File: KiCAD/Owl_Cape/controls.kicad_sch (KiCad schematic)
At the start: 3 parts, among them J17 OLED, SW1 Enter BTN, SW2 Down BTN

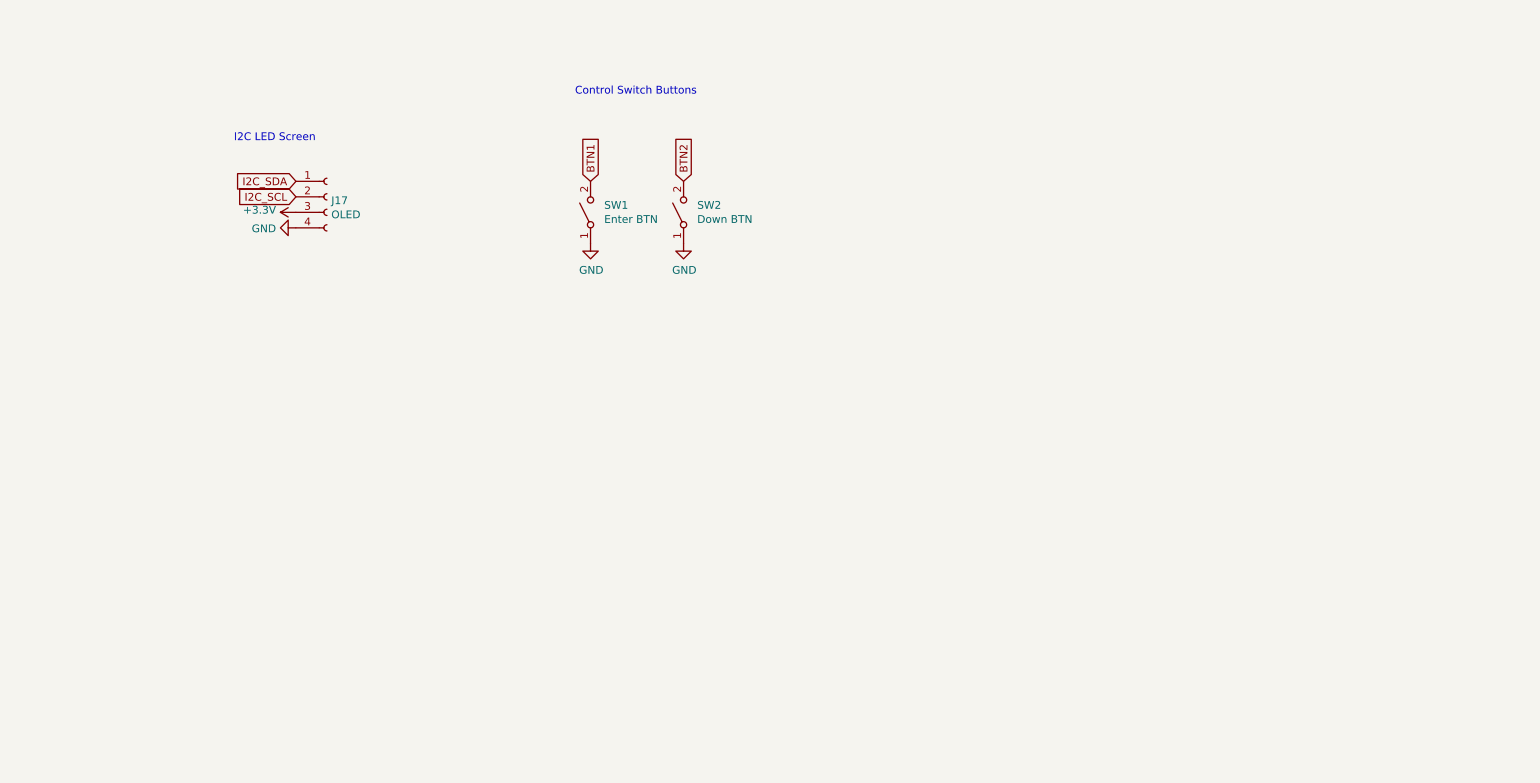
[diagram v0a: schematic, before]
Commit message: started routing cu
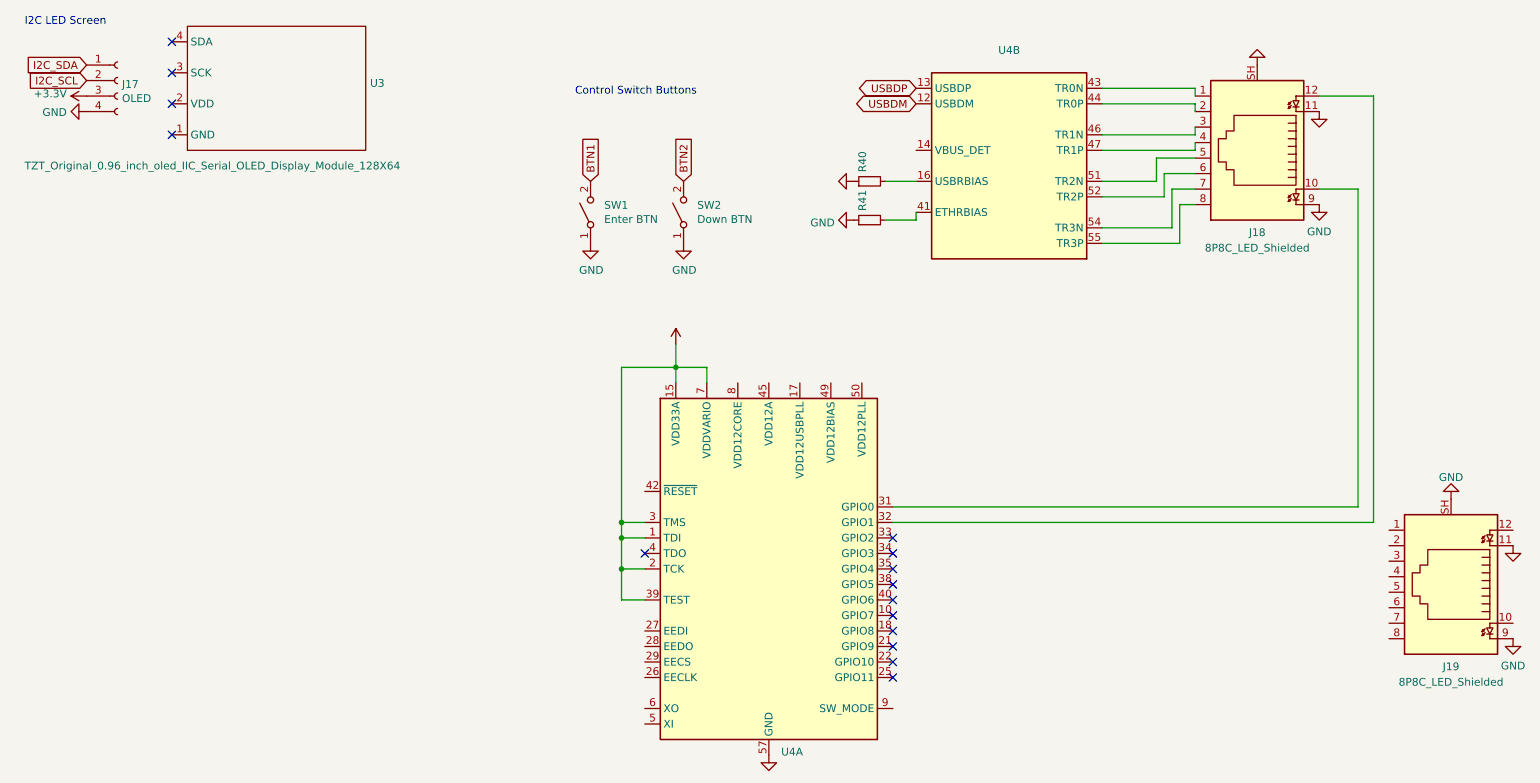
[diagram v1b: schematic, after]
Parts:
- added J18, J19: 8P8C_LED_Shielded, Connector_RJ:RJ45_BEL_SS74301-00x_Vertical, symbol Connector:8P8C_LED_Shielded
- added R40, R41: (no value), symbol Device:R_Small
- added U3: TZT_Original_0.96_inch_oled_IIC_Serial_OLED_Displ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, Stuart_BESPOKE:TZT_0.96inch_OLED, symbol Stuarts_BESPOKE:TZT_Original_0.96_inch_oled_IIC_Serial_OLED_Display_Module_128X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
- added U4: (no value), symbol Interface_Ethernet:LAN7500-ABJZ
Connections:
- net +3V3: now also U4.1 (TDI), U4.15 (VDD33A), U4.19 (VDDVARIO), U4.2 (TCK), U4.24 (VDDVARIO), U4.3 (TMS), U4.37 (VDDVARIO), U4.39 (TEST), U4.7 (VDDVARIO)
- net GND: now also J18.11, J18.9, J18.SH, J19.11, J19.9, J19.SH, R40.1, R41.1, U4.57 (GND)
- new net: R40.2, U4.16 (USBRBIAS)
- new net: U4.11 (VDD12CORE), U4.20 (VDD12CORE), U4.23 (VDD12CORE), U4.30 (VDD12CORE), U4.36 (VDD12CORE), U4.8 (VDD12CORE)
- new net: J18.10, U4.31 (GPIO0)
- new net: J18.12, U4.32 (GPIO1)
- new net: U4.45 (VDD12A), U4.48 (VDD12A), U4.53 (VDD12A), U4.56 (VDD12A)
- new net: R41.2, U4.41 (ETHRBIAS)
- new net: J18.1, U4.43 (TR0N)
- new net: J18.2, U4.44 (TR0P)
- new net: J18.3, U4.46 (TR1N)
- new net: J18.4, U4.47 (TR1P)
- new net: J18.5, U4.51 (TR2N)
- new net: J18.6, U4.52 (TR2P)
- new net: J18.7, U4.54 (TR3N)
- new net: J18.8, U4.55 (TR3P)
- new net USBDM: U4.12 (USBDM)
- new net USBDP: U4.13 (USBDP)
- no-connect marks 0 -> 15
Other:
- moved on the sheet: J17
